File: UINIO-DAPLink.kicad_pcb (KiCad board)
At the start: 2 copper layers, 94 x 30 mm, 52 parts, among them J1 扩展板串口 & 电源输出, J2 扩展板 JTAG 输出, J3 JTAG_nTRST 跳线选择, J4 3.3V 跳线选择, J5 扩展板 SWD 输入, J6 DAPLink 固件下载接口, J7 SWD 下载输出, U1 ME6211C33M5G, U2 STM32F103C8T6, Y1 8MHz

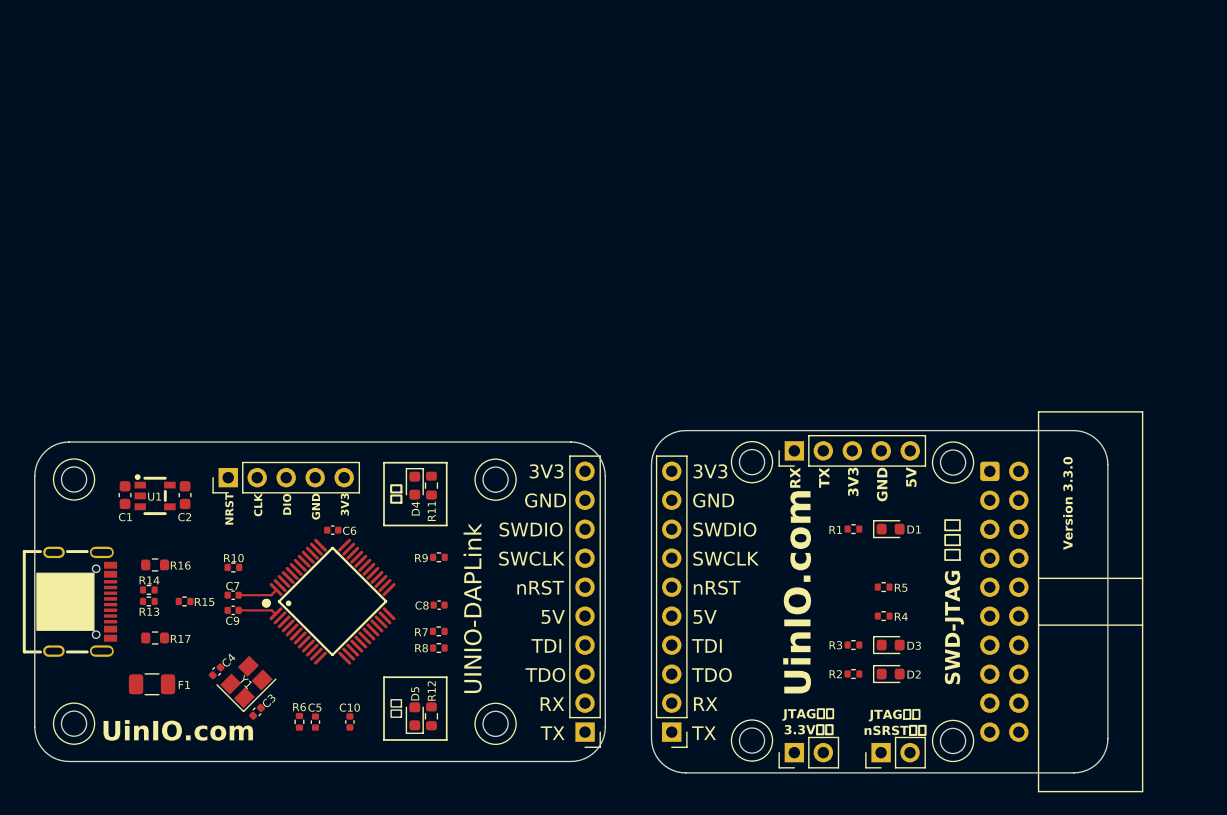
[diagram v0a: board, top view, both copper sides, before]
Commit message: update
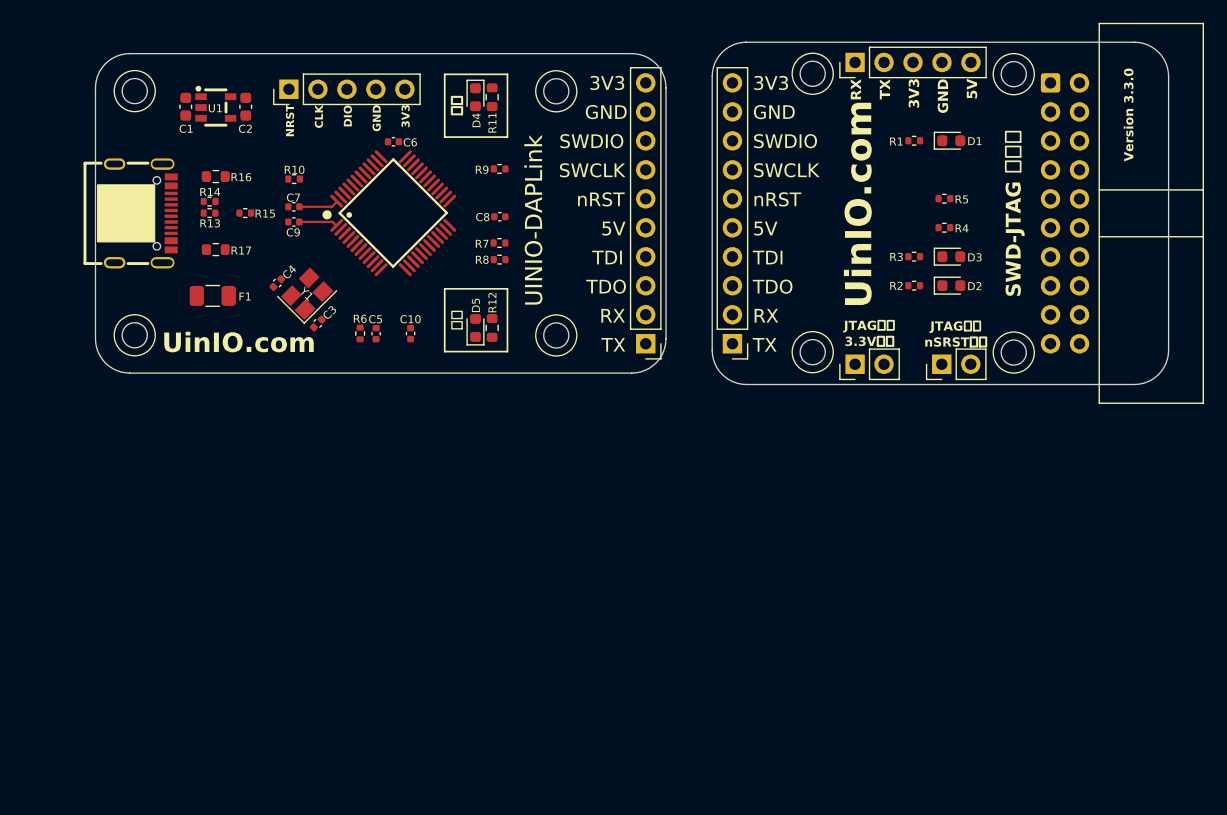
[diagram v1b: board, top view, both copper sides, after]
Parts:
- moved C7 34.5 mm to (116.7, 102.1)
- moved HOLE** 34.5 mm to (102.8, 113.3)
- moved C2 34.5 mm to (112.5, 93.3)
- moved C6 34.5 mm to (125.4, 96.4)
- moved R13 34.5 mm to (109.3, 102.6)
- moved R15 34.5 mm to (112.4, 102.6)
- moved R4 34.5 mm to (173.7, 103.9)
- moved USB1 34.5 mm to (103.5, 102.6)
- moved C1 34.5 mm to (107.2, 93.3)
- moved C10 34.5 mm to (126.9, 113.2)
- moved C3 34.5 mm to (118.8, 112.3)
- moved C8 34.5 mm to (134.7, 102.9)
- moved D1 34.5 mm to (174.3, 96.3)
- moved HOLE** 34.5 mm to (179.8, 114.8)
- moved HOLE** 34.5 mm to (162.2, 114.8)
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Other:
- board size 94 x 30 mm -> 94.1 x 30 mm
